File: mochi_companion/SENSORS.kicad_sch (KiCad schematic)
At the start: 9 parts, among them U12 BME680, U2 RV-3028-C7

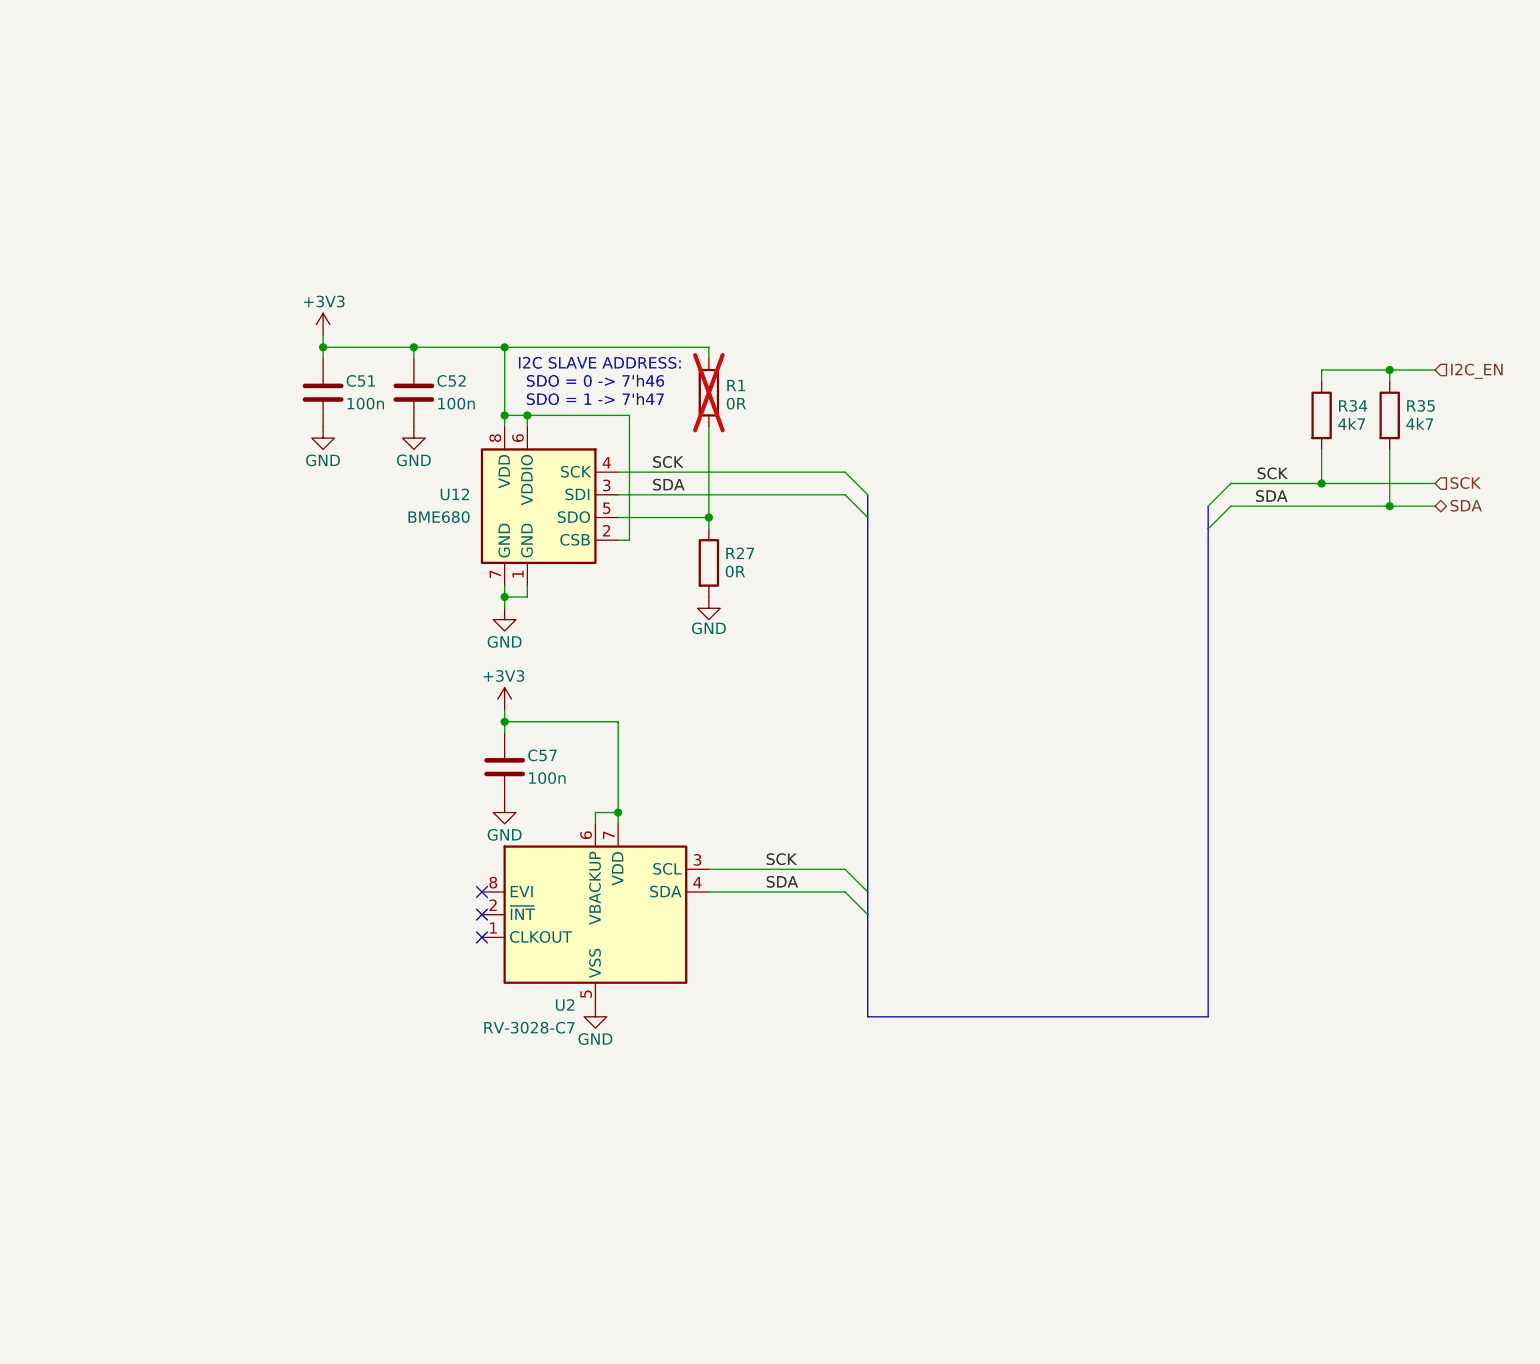
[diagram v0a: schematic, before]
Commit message: 250712_0041
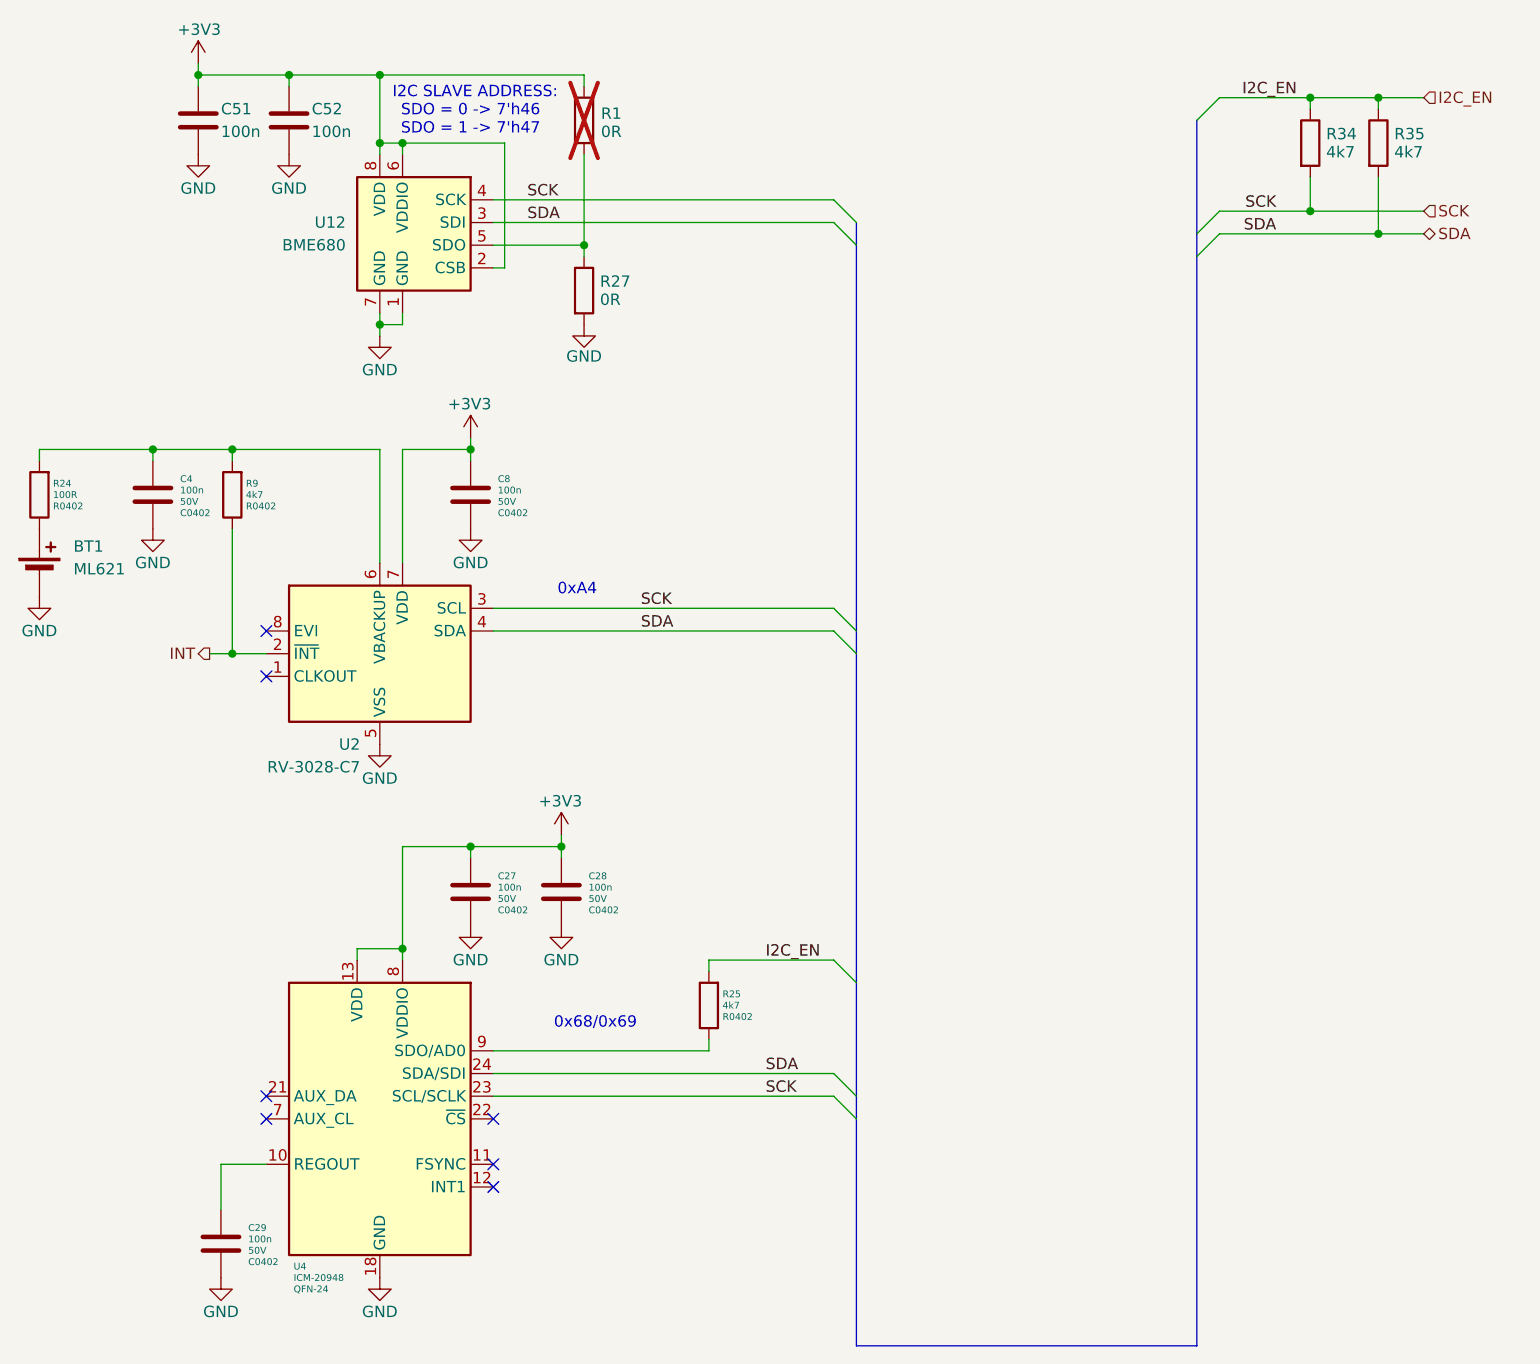
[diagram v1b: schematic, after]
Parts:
- removed C57: 100n, Capacitor_SMD:C_0402_1005Metric, symbol Device:C
- added BT1: ML621, symbol Device:Battery_Cell
- added C27, C28, C29, C4, C8: 100n, Capacitor_SMD:C_0402_1005Metric, symbol Device:C
- added R24: 100R, PCM_Resistor_SMD_AKL:R_0402_1005Metric, symbol Device:R
- added R25, R9: 4k7, PCM_Resistor_SMD_AKL:R_0402_1005Metric, symbol Device:R
- added U4: ICM-20948, Sensor_Motion:InvenSense_QFN-24_3x3mm_P0.4mm, symbol Sensor_Motion:ICM-20948
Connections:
- net +3V3: now also C27.1, C28.1, C8.1, U4.13 (VDD), U4.8 (VDDIO); no longer U2.6 (VBACKUP)
- net GND: now also BT1.2 (-), C27.2, C28.2, C29.2, C4.2, C8.2, U4.18 (GND), U4.20 (GND)
- net I2C_EN: now also R25.2
- net SCK: now also U4.23 (SCL/SCLK)
- net SDA: now also U4.24 (SDA/SDI)
- net INT: now reaches U2.2 (~{INT})
- net INT: now also R9.1
- new net: C4.1, R24.2, R9.2, U2.6 (VBACKUP)
- new net: BT1.1 (+), R24.1
- new net: C29.1, U4.10 (REGOUT)
- new net: R25.1, U4.9 (SDO/AD0)
- no-connect marks 3 -> 7
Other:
- note added: "0x68/0x69"
- note added: "0xA4"
- moved on the sheet: C51, C52, R1, R27, R34, R35, U12, U2
